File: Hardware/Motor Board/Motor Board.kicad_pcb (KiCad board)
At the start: 2 copper layers, 43 parts, among them J1 Input Board, J2 Speed, J3 Power, J4 Indicator LED, J5 Auto / Fwd / Rev, J6 Direction LED (Bi-Color), J7 Motor, J8 KBLC-240D, J9 KBSI-240D, K1 SRD-05VDC-SL-C, K2 SRD-05VDC-SL-C, K3 SRD-05VDC-SL-C, K4 SRD-05VDC-SL-C, K5 SRD-05VDC-SL-C, Q1 2N2222, Q2 2N2222, Q3 2N2222, Q4 2N2222, Q5 2N2222

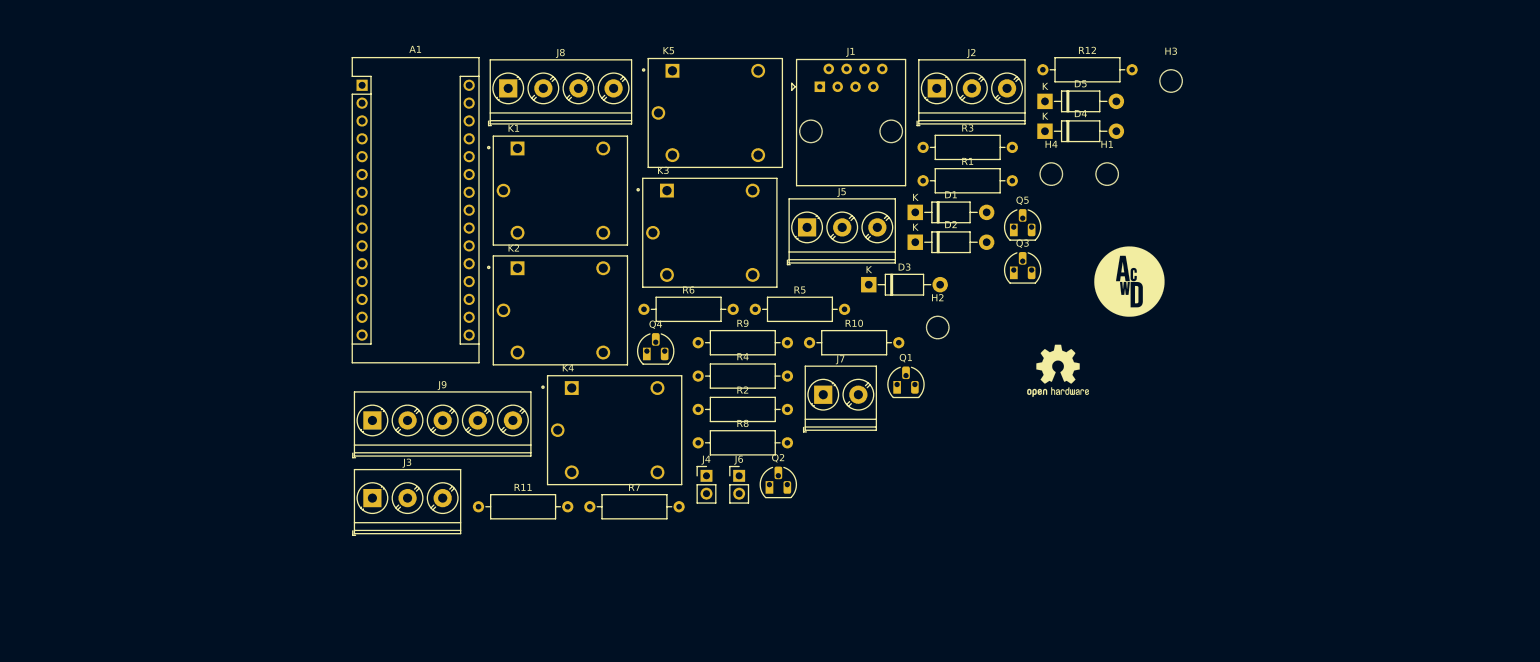
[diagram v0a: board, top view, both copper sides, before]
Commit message: Rev A boards ordered
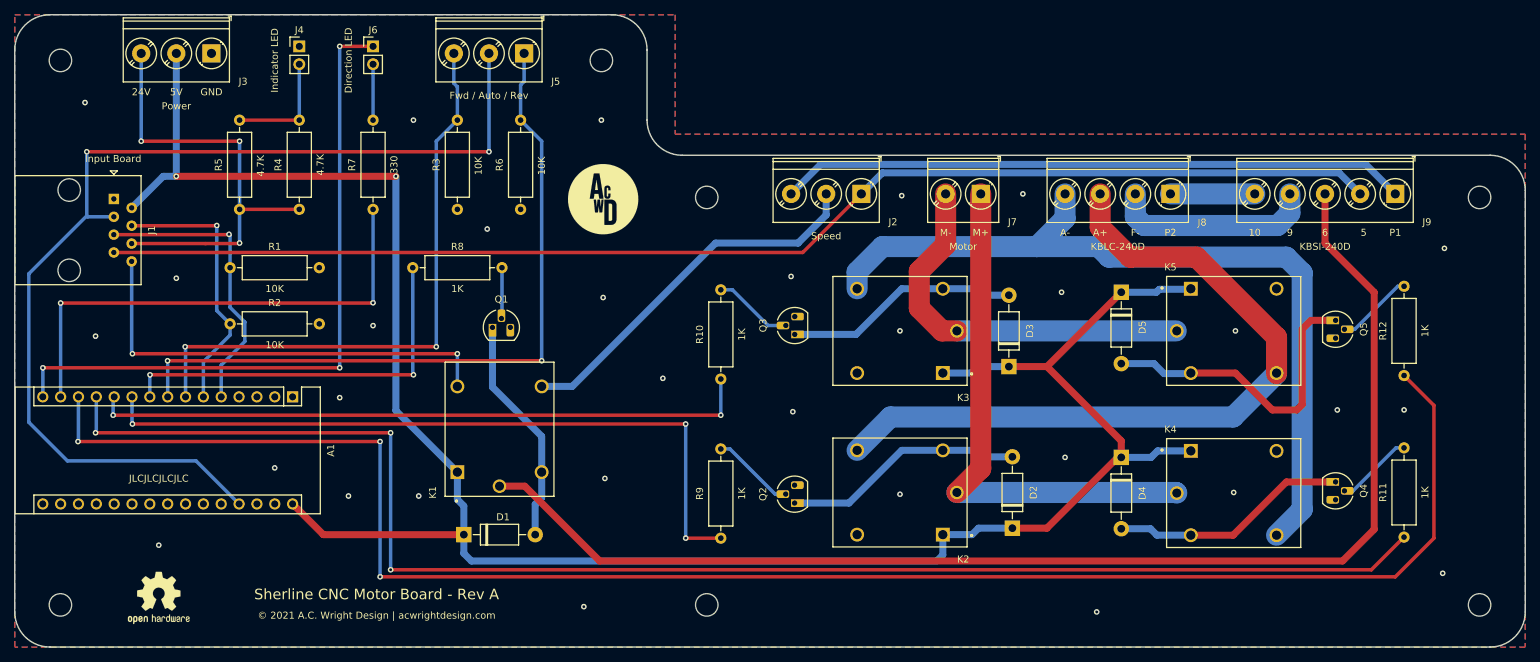
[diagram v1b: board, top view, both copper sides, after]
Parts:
- added H5: MountingHole, MountingHole:MountingHole_3.2mm_M3, F.Cu at (250.5, 82.0)
- added H6: MountingHole, MountingHole:MountingHole_3.2mm_M3, F.Cu at (140.5, 82.0)
- added H7: MountingHole, MountingHole:MountingHole_3.2mm_M3, F.Cu at (125.5, 62.5)
- J5: value Auto / Fwd / Rev -> Fwd / Auto / Rev
- J6: value Direction LED (Bi-Color) -> Direction LED
- moved H1 149.9 mm to (48.5, 62.5)
- moved J9 149.1 mm to (238.5, 81.5), turned to 180 degrees
- moved REF** 132.0 mm to (62.5, 139.0)
- moved R11 131.8 mm to (239.8, 130.3), turned to 90 degrees
- moved H2 131.0 mm to (48.5, 140.0)
- moved J1 101.8 mm to (56.1, 82.2), turned to -90 degrees
- moved Q4 99.8 mm to (230.0, 122.5), turned to -90 degrees
- moved H3 99.6 mm to (140.5, 140.0)
- moved R1 99.4 mm to (72.7, 92.0)
- moved J8 95.4 mm to (206.5, 81.5), turned to 180 degrees
- moved K4 88.6 mm to (215.5, 124.1)
- moved H4 86.5 mm to (250.5, 140.0)
- moved J4 84.2 mm to (82.5, 60.5)
- moved J6 80.3 mm to (93.0, 60.5)
- moved K5 80.0 mm to (215.5, 101.0)
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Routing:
- net VIN: track 0.00 -> 310.7 mm, vias 0 -> 2
- net D10: track 0.00 -> 245.8 mm, vias 0 -> 3
- net D9: track 0.00 -> 212.8 mm, vias 0 -> 3
- net K5: track 0.00 -> 183.3 mm
- net K6: track 0.00 -> 181.4 mm
- net 5V: track 0.00 -> 151.8 mm, vias 0 -> 2
- net A-: track 0.00 -> 116.8 mm
- net A+: track 0.00 -> 105.7 mm
- net D7: track 0.00 -> 103.9 mm, vias 0 -> 3
- net Net-(A1-Pad8): track 0.00 -> 103.6 mm, vias 0 -> 2
- net Net-(A1-Pad15): track 0.00 -> 96.9 mm, vias 0 -> 3
- net D8: track 0.00 -> 94.3 mm, vias 0 -> 2
- net P1: track 0.00 -> 89.5 mm
- net Net-(A1-Pad7): track 0.00 -> 86.1 mm, vias 0 -> 2
- net M+: track 0.00 -> 75.2 mm
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- added copper zone on B.Cu, net GND
- added copper zone on F.Cu, net GND
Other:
- board outline added: 215 x 90 mm
- board text added: "10"
- board text added: "24V"
- board text added: "5"
- board text added: "5V"
- board text added: "6"
- board text added: "9"
- board text added: "A+"
- board text added: "A-"
- board text added: "F-"
- board text added: "GND"
- board text added: "JLCJLCJLCJLC"
- board text added: "M+"
- board text added: "M-"
- board text added: "P1"
- board text added: "P2"
- board text added: "Sherline CNC Motor Board - Rev A"
- board text added: "© 2021 A.C. Wright Design | acwrightdesign.com"
